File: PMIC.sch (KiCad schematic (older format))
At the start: 71 parts, among them U4 CSD86330Q3D, U5 LMR62014XMF_NOPB, U6 CSD86330Q3D, U8 TPS65086100

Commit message: Update libs
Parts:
- R10, R11, R12, R123, R14, R15, R16, R5, R6: footprint antmicro-footprints:0201-res -> arvsom-footprints:0201-res; symbol antmicroResistorsmisc:R_0R_0201 -> arvsom:R_0R_0201
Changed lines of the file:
@@
 	4625 4775 5275 4775
 $Comp
-L antmicroResistorsmisc:R_0R_0201 R5
+L arvsom:R_0R_0201 R5
 U 1 1 60A1EF73
 P 5425 4775
 F 0 "R5" H 5250 4825 60  0000 C CNN
 F 1 "R_0R_0201" H 5425 4625 60  0001 C CNN
-F 2 "antmicro-footprints:0201-res" H 5625 4975 60  0001 L CNN
+F 2 "arvsom-footprints:0201-res" H 5625 4975 60  0001 L CNN
 F 3 "" H 5425 4775 50  0001 C CNN
 F 4 "VISHAY" H 5625 5175 60  0001 L CNN "Manufacturer"
@@
 $EndComp
 $Comp
-L antmicroResistorsmisc:R_0R_0201 R6
+L arvsom:R_0R_0201 R6
 U 1 1 60A26BB5
 P 5425 4875
 F 0 "R6" H 5250 4925 60  0000 C CNN
 F 1 "R_0R_0201" H 5425 4725 60  0001 C CNN
-F 2 "antmicro-footprints:0201-res" H 5625 5075 60  0001 L CNN
+F 2 "arvsom-footprints:0201-res" H 5625 5075 60  0001 L CNN
 F 3 "" H 5425 4875 50  0001 C CNN
 F 4 "VISHAY" H 5625 5275 60  0001 L CNN "Manufacturer"
@@
 $EndComp
 $Comp
-L antmicroResistorsmisc:R_0R_0201 R123
+L arvsom:R_0R_0201 R123
 U 1 1 60A2A03C
 P 5425 5575
 F 0 "R123" H 5375 5675 60  0000 C CNN
 F 1 "R_0R_0201" H 5425 5425 60  0001 C CNN
-F 2 "antmicro-footprints:0201-res" H 5625 5775 60  0001 L CNN
+F 2 "arvsom-footprints:0201-res" H 5625 5775 60  0001 L CNN
 F 3 "" H 5425 5575 50  0001 C CNN
 F 4 "VISHAY" H 5625 5975 60  0001 L CNN "Manufacturer"
@@
 $EndComp
 $Comp
-L antmicroResistorsmisc:R_0R_0201 R10
+L arvsom:R_0R_0201 R10
 U 1 1 60A468A9
 P 8500 3775
 F 0 "R10" H 8275 3825 60  0000 C CNN
 F 1 "R_0R_0201" H 8500 3625 60  0001 C CNN
-F 2 "antmicro-footprints:0201-res" H 8700 3975 60  0001 L CNN
+F 2 "arvsom-footprints:0201-res" H 8700 3975 60  0001 L CNN
 F 3 "" H 8500 3775 50  0001 C CNN
 F 4 "VISHAY" H 8700 4175 60  0001 L CNN "Manufacturer"
@@
 $EndComp
 $Comp
-L antmicroResistorsmisc:R_0R_0201 R11
+L arvsom:R_0R_0201 R11
 U 1 1 60A4B370
 P 8500 3875
 F 0 "R11" H 8275 3925 60  0000 C CNN
 F 1 "R_0R_0201" H 8500 3725 60  0001 C CNN
-F 2 "antmicro-footprints:0201-res" H 8700 4075 60  0001 L CNN
+F 2 "arvsom-footprints:0201-res" H 8700 4075 60  0001 L CNN
 F 3 "" H 8500 3875 50  0001 C CNN
 F 4 "VISHAY" H 8700 4275 60  0001 L CNN "Manufacturer"
@@
 $EndComp
 $Comp
-L antmicroResistorsmisc:R_0R_0201 R12
+L arvsom:R_0R_0201 R12
 U 1 1 60A4C09F
 P 8500 4075
 F 0 "R12" H 8275 4125 60  0000 C CNN
 F 1 "R_0R_0201" H 8500 3925 60  0001 C CNN
-F 2 "antmicro-footprints:0201-res" H 8700 4275 60  0001 L CNN
+F 2 "arvsom-footprints:0201-res" H 8700 4275 60  0001 L CNN
 F 3 "" H 8500 4075 50  0001 C CNN
 F 4 "VISHAY" H 8700 4475 60  0001 L CNN "Manufacturer"
@@
 $EndComp
 $Comp
-L antmicroResistorsmisc:R_0R_0201 R14
+L arvsom:R_0R_0201 R14
 U 1 1 60A523FE
 P 8500 5375
 F 0 "R14" H 8275 5425 60  0000 C CNN
 F 1 "R_0R_0201" H 8500 5225 60  0001 C CNN
-F 2 "antmicro-footprints:0201-res" H 8700 5575 60  0001 L CNN
+F 2 "arvsom-footprints:0201-res" H 8700 5575 60  0001 L CNN
 F 3 "" H 8500 5375 50  0001 C CNN
 F 4 "VISHAY" H 8700 5775 60  0001 L CNN "Manufacturer"
@@
 $EndComp
 $Comp
-L antmicroResistorsmisc:R_0R_0201 R15
+L arvsom:R_0R_0201 R15
 U 1 1 60A56682
 P 8500 5475
 F 0 "R15" H 8275 5525 60  0000 C CNN
 F 1 "R_0R_0201" H 8500 5325 60  0001 C CNN
-F 2 "antmicro-footprints:0201-res" H 8700 5675 60  0001 L CNN
+F 2 "arvsom-footprints:0201-res" H 8700 5675 60  0001 L CNN
 F 3 "" H 8500 5475 50  0001 C CNN
 F 4 "VISHAY" H 8700 5875 60  0001 L CNN "Manufacturer"
@@
 $EndComp
 $Comp
-L antmicroResistorsmisc:R_0R_0201 R16
+L arvsom:R_0R_0201 R16
 U 1 1 60A57367
 P 8500 5675
 F 0 "R16" H 8275 5725 60  0000 C CNN
 F 1 "R_0R_0201" H 8500 5525 60  0001 C CNN
-F 2 "antmicro-footprints:0201-res" H 8700 5875 60  0001 L CNN
+F 2 "arvsom-footprints:0201-res" H 8700 5875 60  0001 L CNN
 F 3 "" H 8500 5675 50  0001 C CNN
 F 4 "VISHAY" H 8700 6075 60  0001 L CNN "Manufacturer"

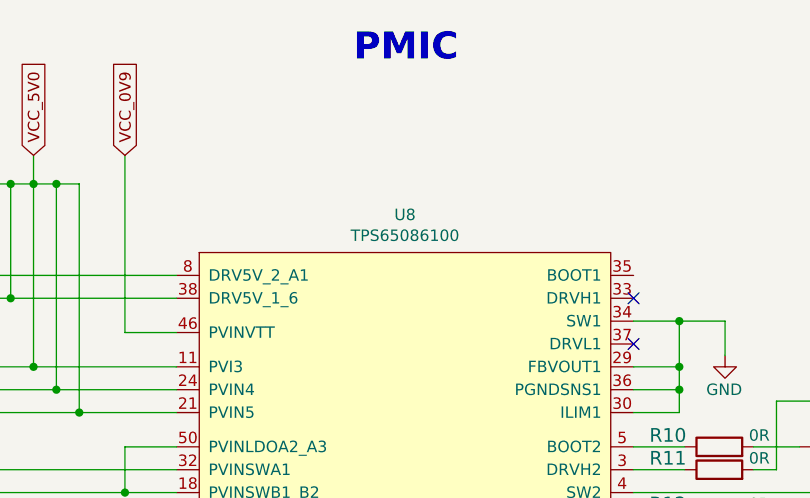
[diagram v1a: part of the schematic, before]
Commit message: Update lib attributes
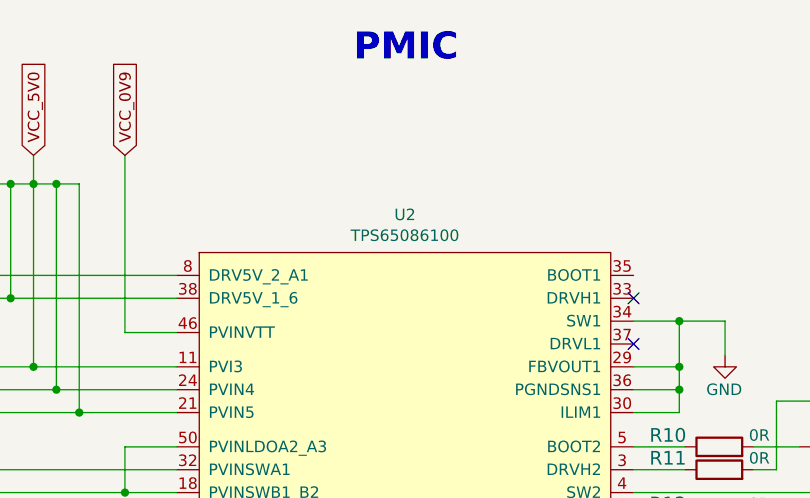
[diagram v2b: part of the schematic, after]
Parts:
- U2: renamed from U8; MPN (none) -> TPS65086100; Manufacturer (none) -> Texas Instruments
- U5: Manufacturer (none) -> Texas Instruments
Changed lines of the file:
@@
 $EndComp
 $Comp
-L arvsom:TPS65086100 U8
+L arvsom:TPS65086100 U2
 U 1 1 606F10CB
 P 6225 2925
-F 0 "U8" H 7125 3090 50  0000 C CNN
+F 0 "U2" H 7125 3090 50  0000 C CNN
 F 1 "TPS65086100" H 7125 2999 50  0000 C CNN
 F 2 "arvsom-footprints:S-PVQFN-N64" H 8025 2975 50  0001 C CNN
 F 3 "" H 6225 2925 50  0001 C CNN
+F 4 "TPS65086100" H 6225 2925 50  0001 C CNN "MPN"
+F 5 "Texas Instruments" H 6225 2925 50  0001 C CNN "Manufacturer"
 	1    6225 2925
 	1    0    0    -1
@@
 F 3 "" H 7000 9775 50  0001 L BNN
 F 4 "LMR62014XMF" H 7000 10253 50  0001 C CNN "MPN"
+F 5 "Texas Instruments" H 7000 9775 50  0001 C CNN "Manufacturer"
 	1    7000 9775
 	1    0    0    -1
